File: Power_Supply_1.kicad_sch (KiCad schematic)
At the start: 13 parts

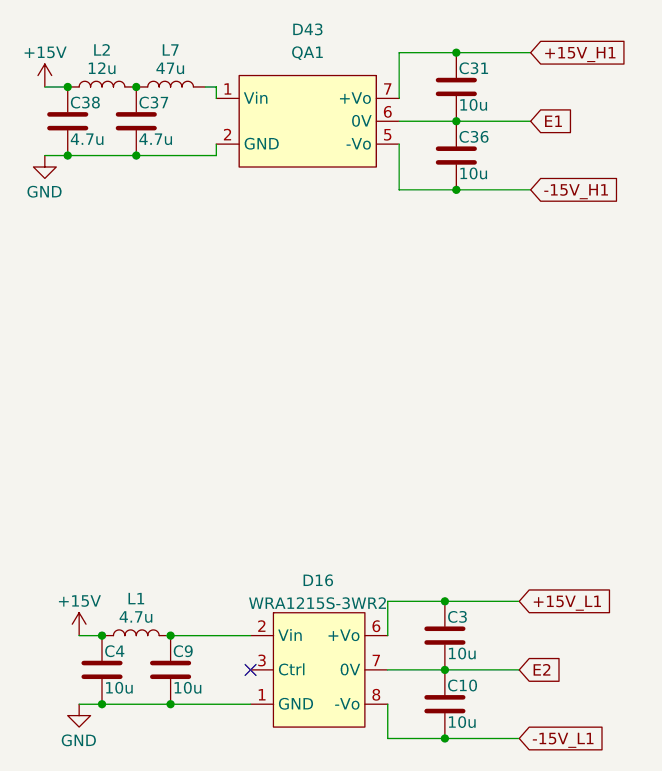
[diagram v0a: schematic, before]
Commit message: VER2.2: все изменения в списке изменений
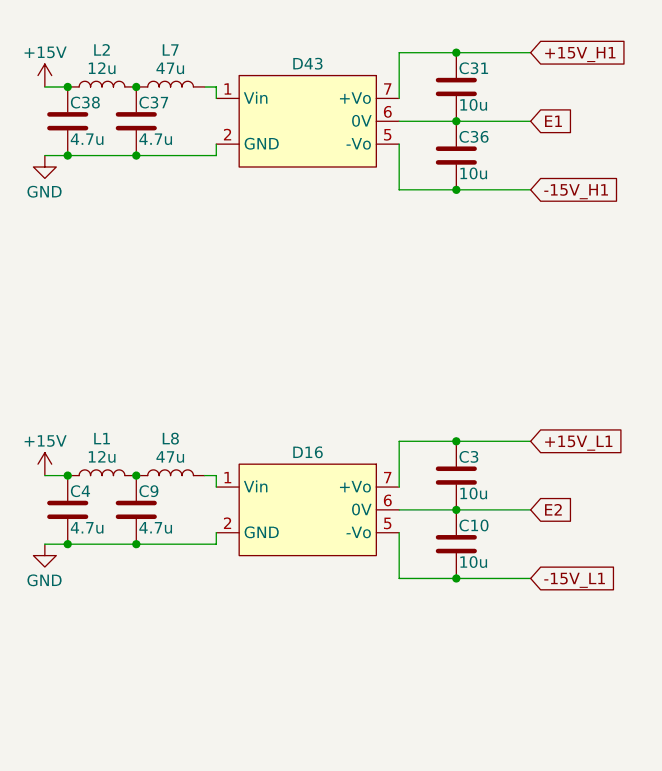
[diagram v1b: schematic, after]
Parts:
- removed D16: WRA1215S-3WR2, Mornsun:WRA_S-3WR2, symbol Morsun:WRA1215S-3WR2
- added D16: ~, DCDC_My:QA, symbol DCDC_My:QA1
- added L8: 47u, Inductor_SMD:L_1812_4532Metric_Pad1.30x3.40mm_HandSolder, symbol Device:L
- C4, C9: value 10u -> 4.7u; footprint Capacitor_SMD:C_1210_3225Metric_Pad1.33x2.70mm_HandSolder -> Capacitor_SMD:C_1206_3216Metric_Pad1.33x1.80mm_HandSolder
- D43: value QA1 -> ~; Description P/N (none) -> DCDC converter; Product Name (none) -> QA1
- L1: value 4.7u -> 12u; footprint Inductor_SMD:L_1812_4532Metric_Pad1.30x3.40mm_HandSolder -> Inductor_SMD:L_1210_3225Metric_Pad1.42x2.65mm_HandSolder; Product Name (none) -> LQH32MN120J23L
- L2: Product Name (none) -> LQH32MN120J23L
- L7: Product Name (none) -> LQH43CN470K03L
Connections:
- net +15V_L1: now also D16.7 (+Vo)
- net -15V_L1: now also D16.5 (-Vo)
- net E2: now also D16.6 (0V)
- net GND: now also D16.2 (GND)
- net at C9.1, L1.2: now also L8.1
- new net: D16.1 (Vin), L8.2
- no-connect marks 1 -> 0
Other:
- moved on the sheet: C10, C3, C4, C9, L1
